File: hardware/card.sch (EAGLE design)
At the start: 74 parts, among them J1 UE27AC54100, J2 B2PS-VH(LF)(SN), J3 MINI-USB-UX60A-MB-5ST, J4 MICROSD, J5 JST_2PIN, U1 ATSAMD21J_QFN, U2 MCP73833, U3 TLV70233DBVR, U4 ATWINC1500_MR210PA, U5 NHD-C12832A1Z-FSW-FBW-3V3, U6 MIC2288YD5-TR, U7 TS3USB221, X3 32.768

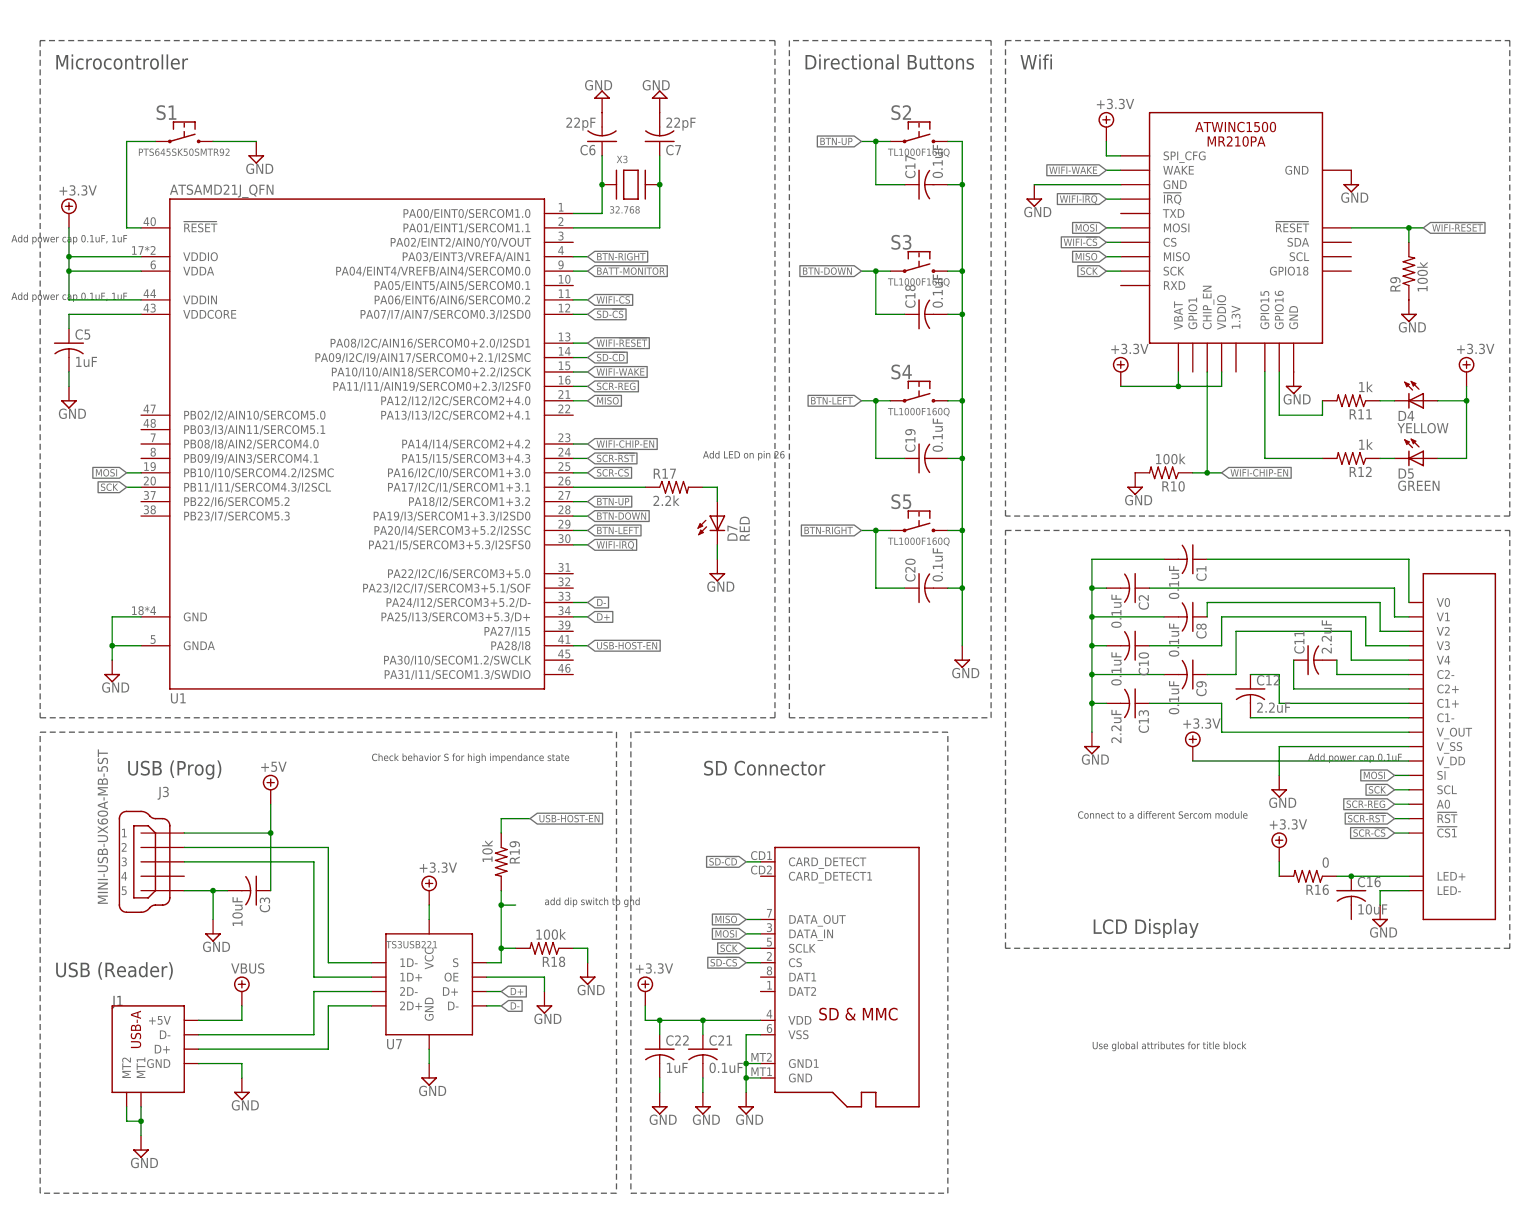
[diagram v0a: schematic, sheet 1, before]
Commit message: Schematic Finished
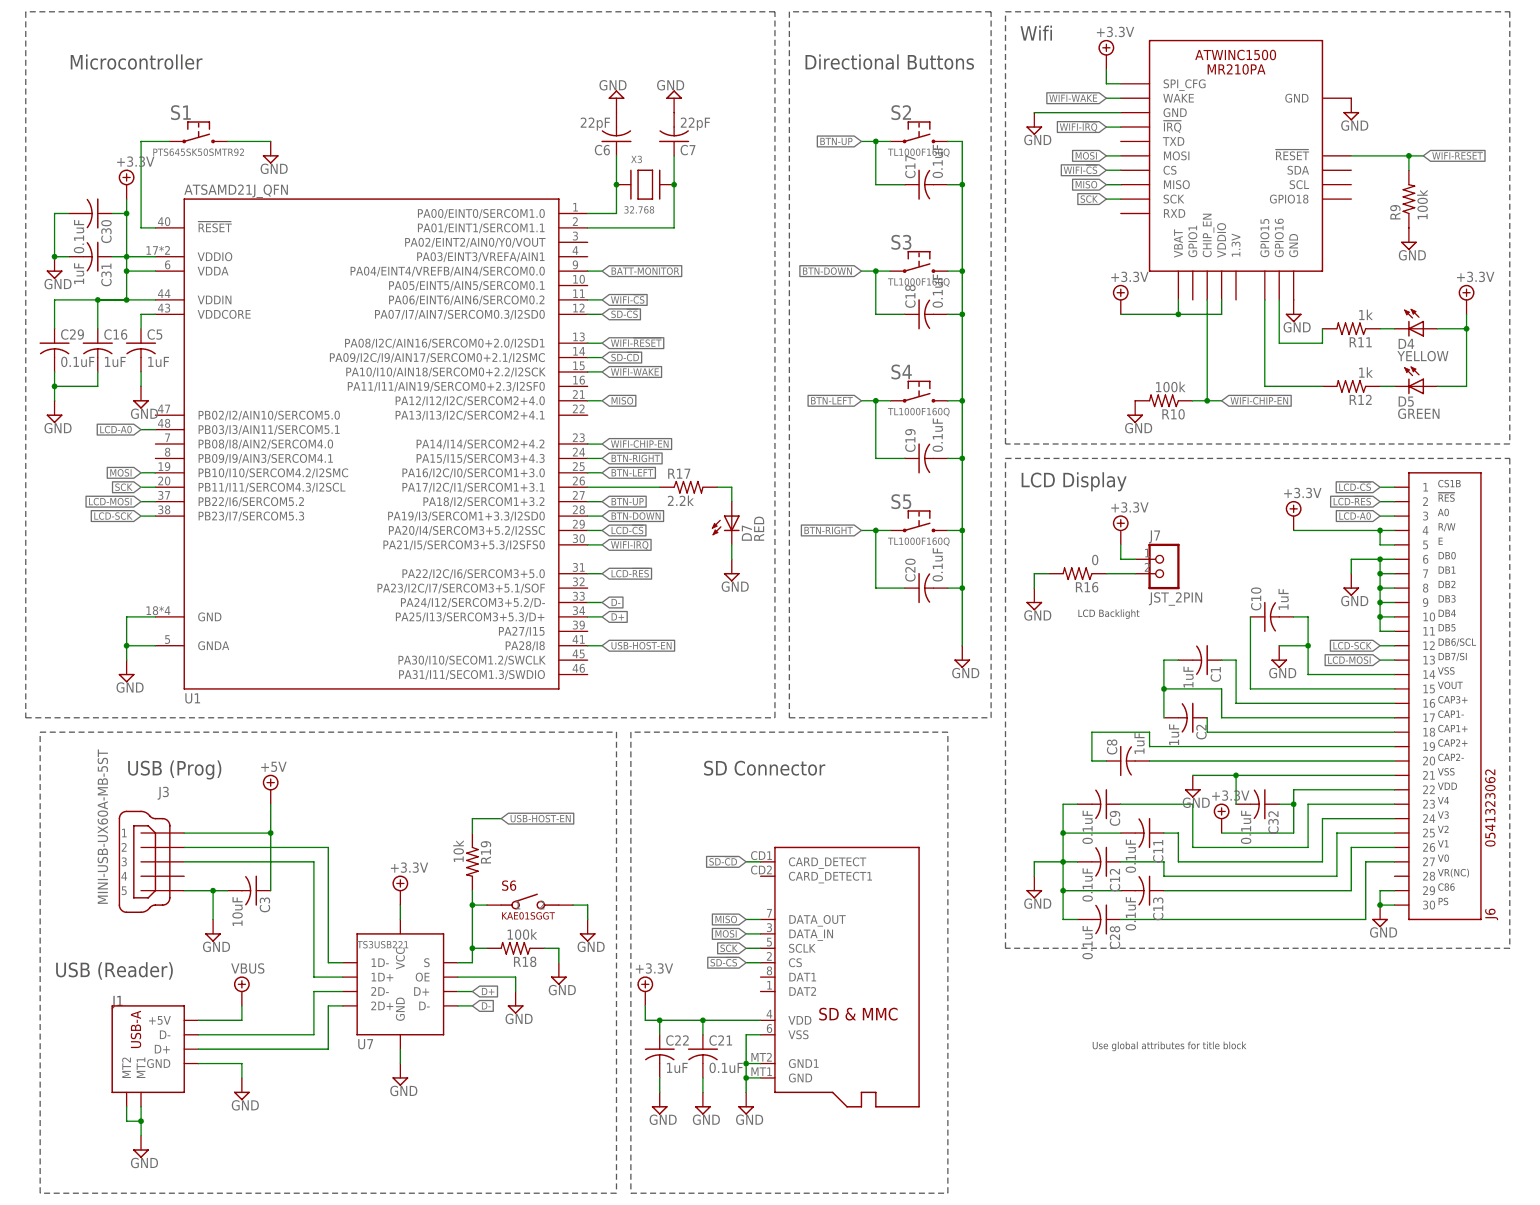
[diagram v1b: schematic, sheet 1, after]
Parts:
- removed U5: NHD-C12832A1Z-FSW-FBW-3V3, CardReader:NHD-C12832A1Z-FSW-FBW-3V3
- added C28, C29, C30, C32: 0.1uF, rcl:C-USC0603
- added C31: 1uF, rcl:C-USC0603
- added J6: 0541323062, CardReader:0541323062
- added J7: JST_2PIN, card:JST_2PIN
- added S6: KAE01SGGT, CardReader:KAE01SGGT
- C1, C10, C2, C8: value 0.1uF -> 1uF
- C11, C12, C13: value 2.2uF -> 0.1uF
- C16: value 10uF -> 1uF
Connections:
- removed net N$11: C16.1, R16.PIN1, U5.LED+
- removed net N$13: R18.PIN2, R19.PIN2, U7.S
- removed net N$19: C1.1, U5.V0
- removed net N$20: C8.1, U5.V2
- removed net N$21: C10.1, U5.V3
- removed net N$22: C2.1, U5.V1
- removed net N$23: C9.1, U5.V4
- removed net N$24: C11.1, U5.C2+
- removed net N$25: C11.2, U5.C2-
- removed net N$26: C13.1, U5.V_OUT
- removed net N$27: C12.1, U5.C1+
- removed net N$28: C12.2, U5.C1-
- removed net SCR-!CS: U1.PA16/I2C/I0/SERCOM1+3.0, U5.!CS1
- removed net SCR-!RST: U1.PA15/I15/SERCOM3+4.3, U5.!RST
- removed net SCR-REG: U1.PA11/I11/AIN19/SERCOM0+2.3/I2SF0, U5.A0
- new net LCD-!CS: J6.1, U1.PA20/I4/SERCOM3+5.2/I2SSC
- new net LCD-!RES: J6.2, U1.PA22/I2C/I6/SERCOM3+5.0
- new net LCD-A0: J6.3, U1.PB03/I3/AIN11/SERCOM5.1
- new net LCD-CA1+: C2.1, J6.18
- new net LCD-CA1-: C1.2, C2.2, J6.17
- new net LCD-CA2+: C8.1, J6.19
- new net LCD-CA2-: C8.2, J6.20
- new net LCD-CA3+: C1.1, J6.16
- new net LCD-K: J7.2, R16.PIN1
- new net LCD-MOSI: J6.13, U1.PB22/I6/SERCOM5.2
- new net LCD-SCK: J6.12, U1.PB23/I7/SERCOM5.3
- new net LCD-V0: C28.1, J6.27
- new net LCD-V1: C13.1, J6.26
- new net LCD-V2: C12.1, J6.25
- new net LCD-V3: C11.1, J6.24
- new net LCD-V4: C9.1, J6.23
- new net LCD-VOUT: C10.1, J6.15
- new net USB-S: R18.PIN2, R19.PIN2, S6.1, U7.S
- net +3.3V: now also C16.1, C29.1, C30.1, C31.1, C32.1, J6.22, J6.4, J6.5, J7.1; no longer R16.PIN2, U5.V_DD
- net BTN-LEFT: now also U1.PA16/I2C/I0/SERCOM1+3.0; no longer U1.PA20/I4/SERCOM3+5.2/I2SSC
- net BTN-RIGHT: now also U1.PA15/I15/SERCOM3+4.3; no longer U1.PA03/EINT3/VREFA/AIN1
- net GND: now also C11.2, C12.2, C16.2, C28.2, C29.2, C30.2, C31.2, C32.2, J6.10, J6.11, J6.14, J6.21, J6.29, J6.30, J6.6, J6.7, J6.8, J6.9, R16.PIN2, S6.2; no longer C1.2, C2.2, C8.2, U5.LED-, U5.V_SS
- net MOSI: no longer U5.SI
- net SCK: no longer U5.SCL
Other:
- note added: "!RES"
- note added: "A0"
- note added: "C86"
- note added: "CAP1+"
- note added: "CAP1-"
- note added: "CAP2+"
- note added: "CAP2-"
- note added: "CAP3+"
- note added: "CS1B"
- note added: "DB0"
- note added: "DB1"
- note added: "DB2"
- note added: "DB3"
- note added: "DB4"
- note added: "DB5"
- note added: "DB6/SCL"
- note added: "DB7/SI"
- note added: "E"
- note added: "LCD Backlight"
- note added: "PS"
- note added: "R/W"
- note added: "V0"
- note added: "V1"
- note added: "V2"
- note added: "V3"
- note added: "V4"
- note added: "VDD"
- note added: "VOUT"
- note added: "VR(NC)"
- note added: "VSS"
- note removed: "Add LED on pin 26"
- note removed: "Add power cap 0.1uF"
- note removed: "Add power cap 0.1uF, 1uF"
- note removed: "Check behavior S for high impendance state"
- note removed: "Connect to a different Sercom module"
- note removed: "add dip switch to gnd"
- moved on the sheet: C1, C10, C11, C12, C13, C16, C2, C5, C6, C7, C8, C9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
